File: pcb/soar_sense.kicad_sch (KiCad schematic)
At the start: 58 parts, among them J1 Conn_02x03_Top_Bottom, J3 Conn_02x02_Top_Bottom, J4 Conn_02x02_Top_Bottom, J5 Conn_02x02_Top_Bottom, J6 Conn_02x03_Top_Bottom, J7 Conn_02x03_Top_Bottom, J8 Conn_01x06, U1 SPX3819M5-L-3-3, U2 STM32F103CBTx, U3 SHT35-DIS, U4 MAX3051, Y1 8MHz

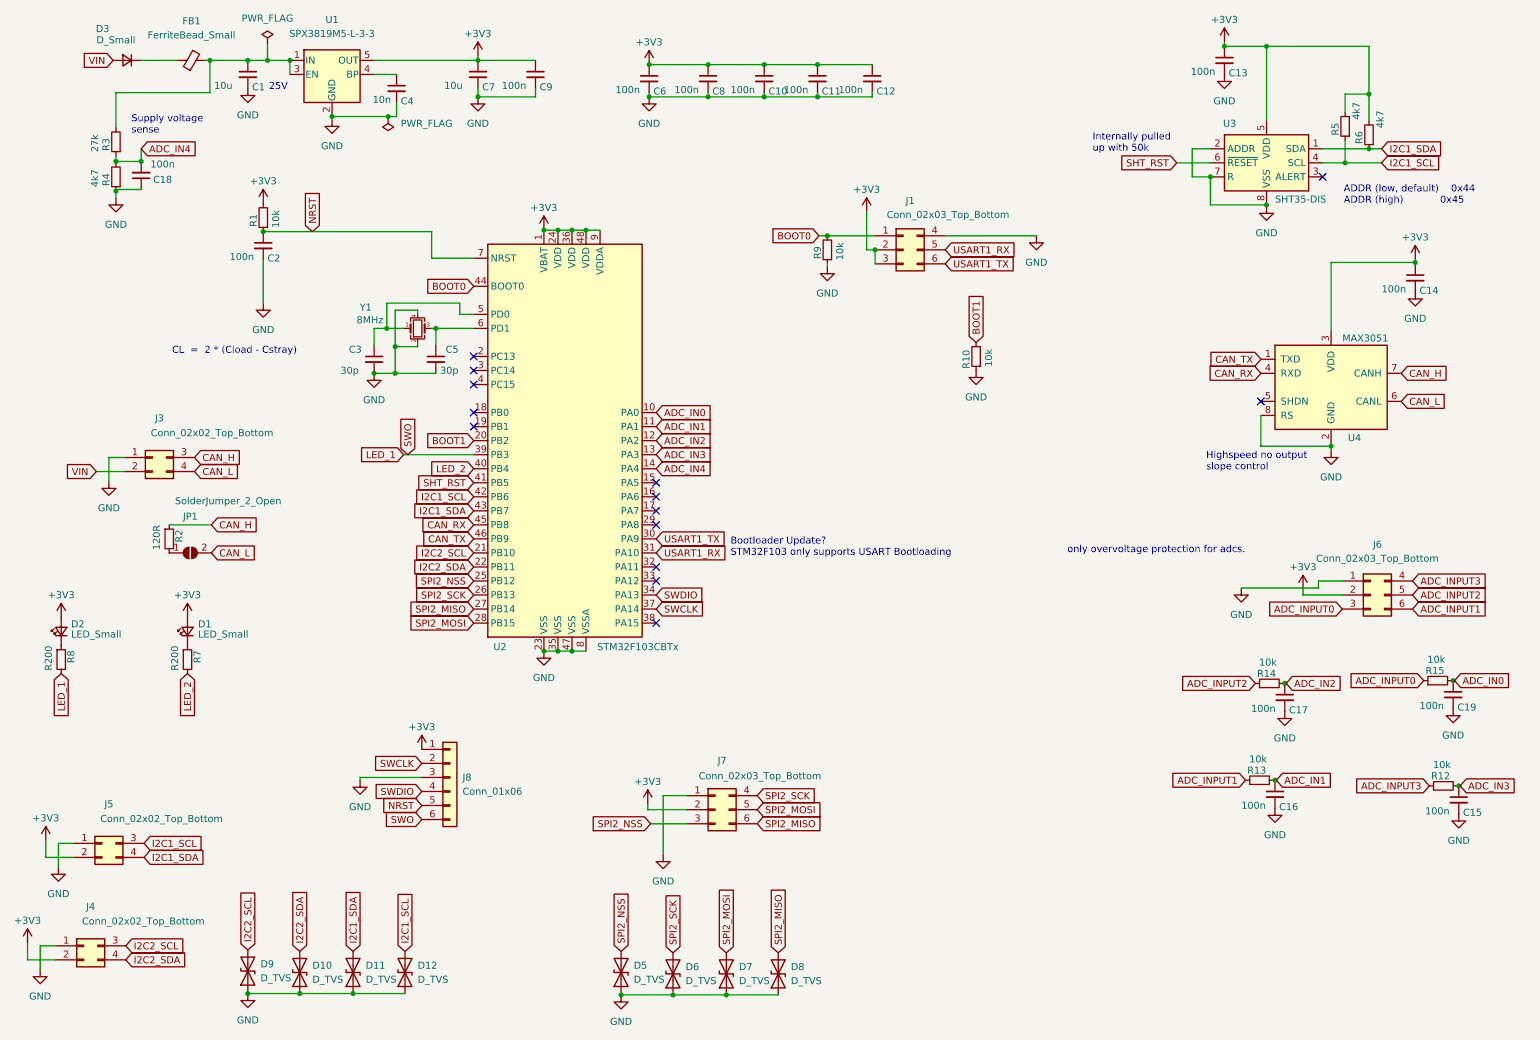
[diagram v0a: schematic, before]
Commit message: updated documentation
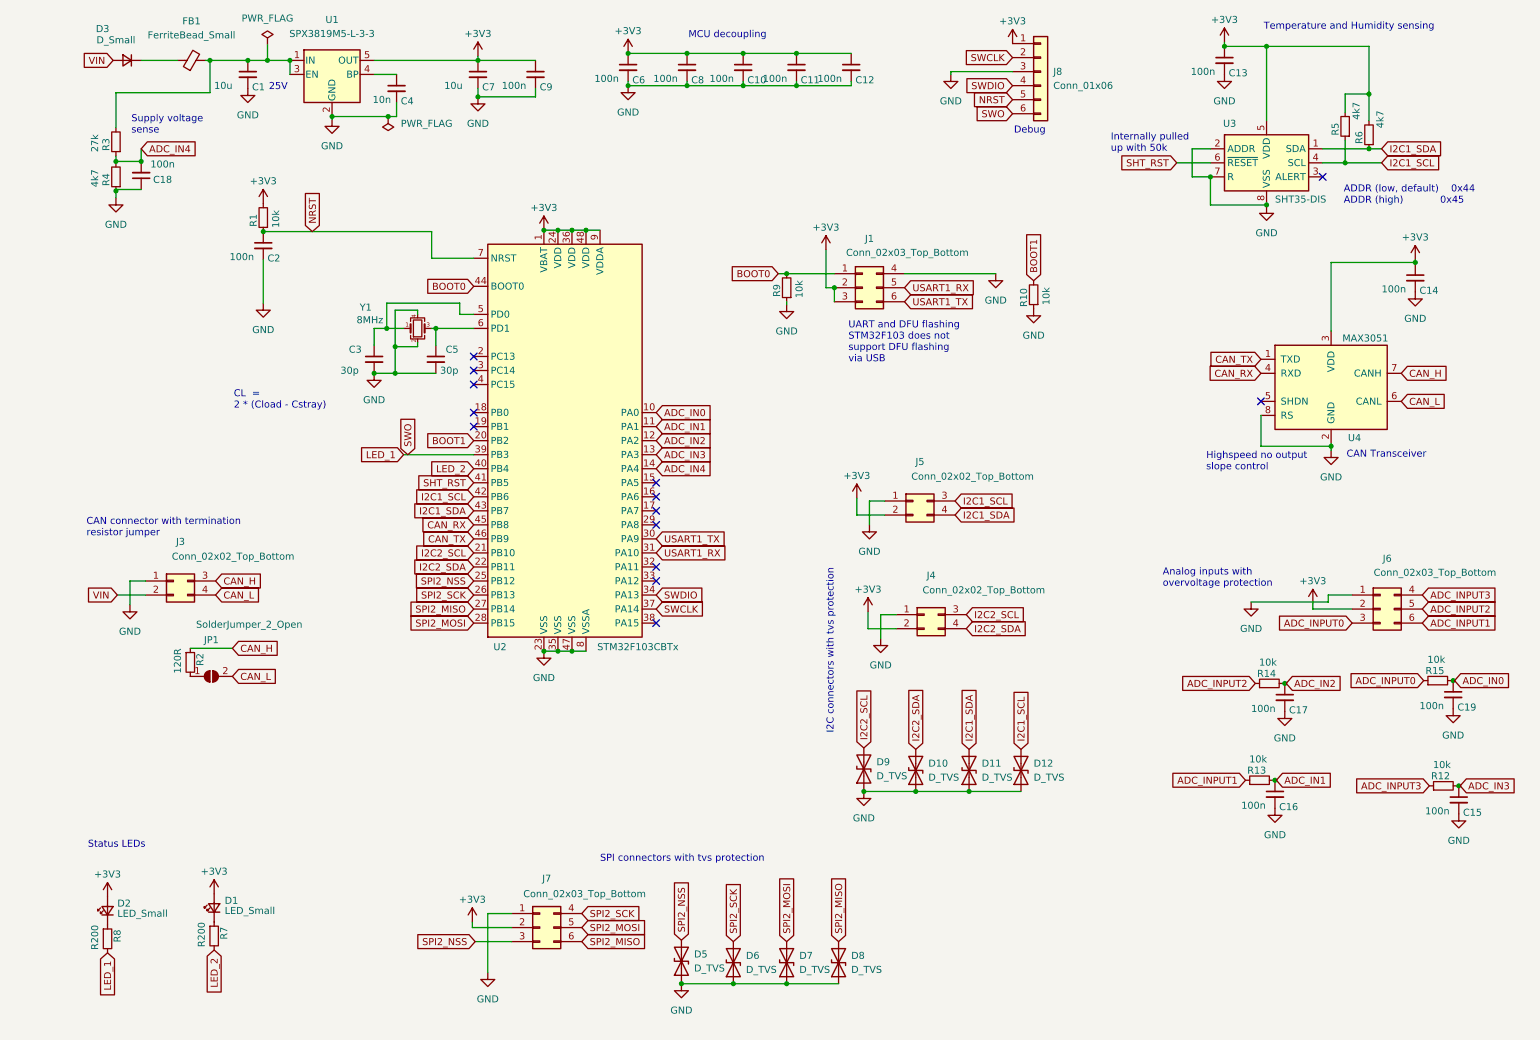
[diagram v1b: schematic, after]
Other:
- note added: "Analog inputs with overvoltage protection"
- note added: "CAN Transceiver"
- note added: "CAN connector with termination resistor jumper"
- note added: "Debug"
- note added: "I2C connectors with tvs protection"
- note added: "MCU decoupling"
- note added: "SPI connectors with tvs protection"
- note added: "Status LEDs"
- note added: "Temperature and Humidity sensing"
- note added: "UART and DFU flashing STM32F103 does not support DFU flashing via USB"
- note removed: "Bootloader Update? STM32F103 only supports USART Bootloading"
- note removed: "only overvoltage protection for adcs."
- title: (none) -> the SOAR SENSE
- moved on the sheet: C10, C11, C12, C6, C8, D1, D10, D11, D12, D2, D5, D6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
